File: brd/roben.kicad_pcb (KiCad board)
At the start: 2 copper layers, 47.6 x 90.2 mm, 45 parts, among them J1 POWER IN, J10 1+, J11 1-, J12 2-, J13 2+, J2 +V, J3 GND, J4 +V, J5 GND, J6 A, J7 B, J8 C, J9 D, U1 TPS54232, U2 SN754410N, U3 Ardunano

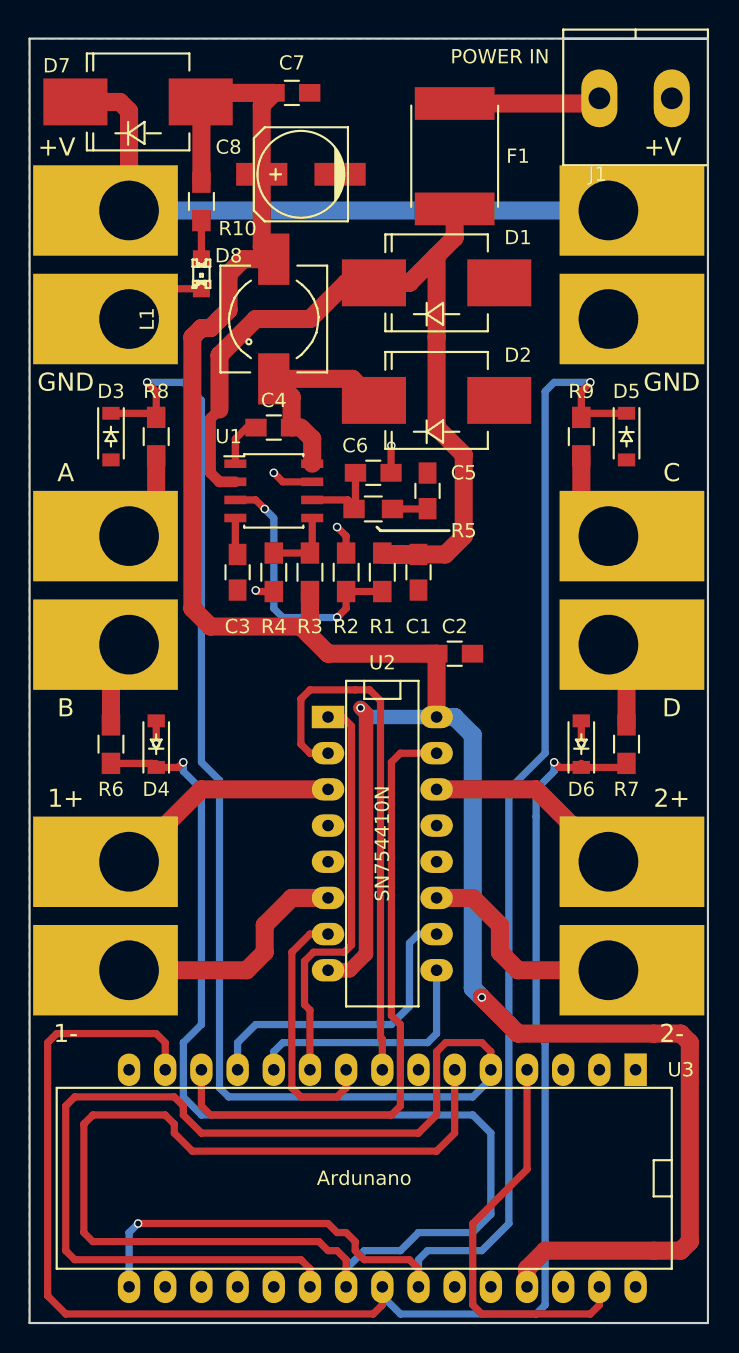
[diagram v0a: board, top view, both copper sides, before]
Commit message: chg: diseñado pcb
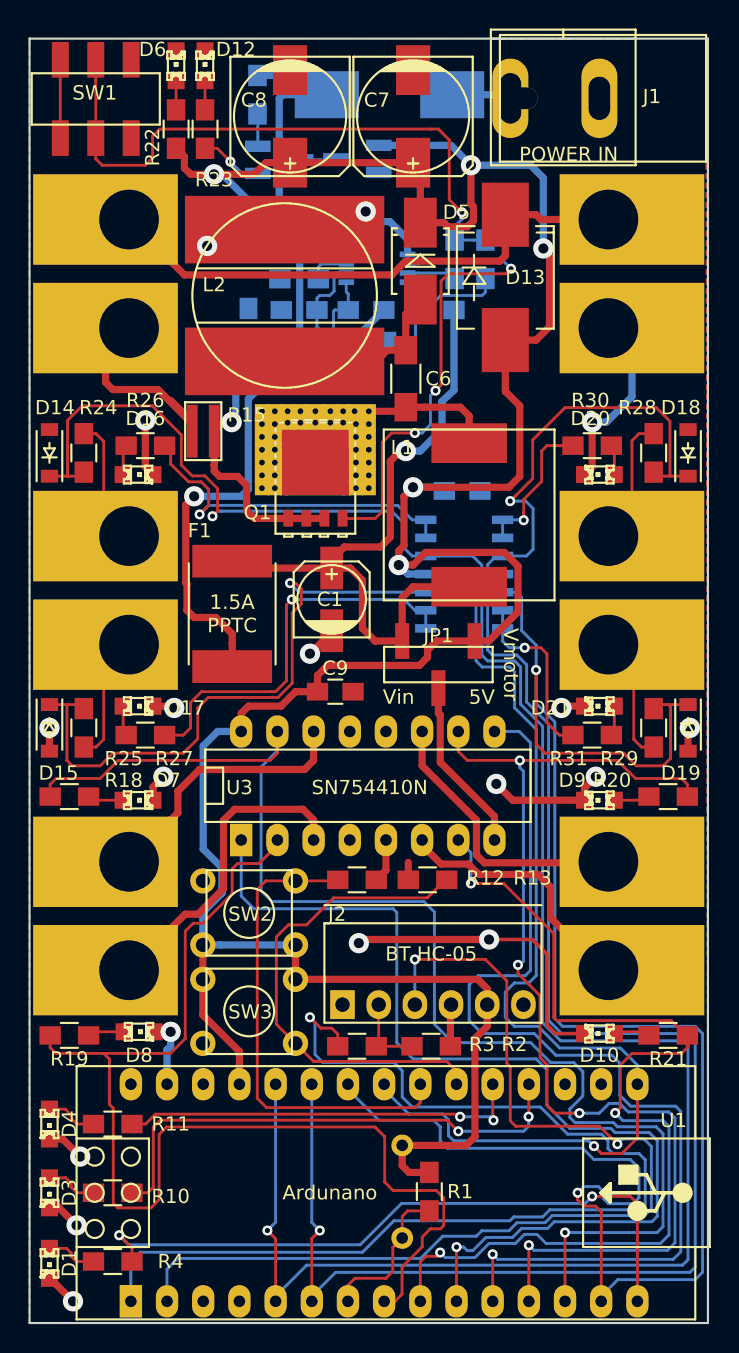
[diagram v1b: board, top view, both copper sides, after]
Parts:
- removed the J7 at (136.5, 93.3)
- removed the J8 at (170.2, 85.7)
- removed the J9 at (170.2, 93.3)
- removed REF**: Symbol_OSHW-Logo_SilkScreen_BIG, Symbols:Symbol_OSHW-Logo_SilkScreen_BIG
- added B: B, Wire_Pads:SolderWirePad_single_2-5mmDrill, F.Cu at (155.6, 81.9)
- added C: C, Wire_Pads:SolderWirePad_single_2-5mmDrill, F.Cu at (153.0, 101.6)
- added C10: 100nF, Capacitors_SMD:C_0805_HandSoldering, B.Cu at (159.9, 82.5)
- added C9: 100nF, Capacitors_SMD:C_0805_HandSoldering, F.Cu at (151.0, 96.6)
- added D: D, Wire_Pads:SolderWirePad_single_2-5mmDrill, F.Cu at (155.6, 111.1)
- added D10: ORANGE, LEDs:LED-0805, F.Cu at (169.5, 120.7)
- added D11: TCMBD914, Housings_SOT-23_SOT-143_TSOT-6:SOT-23_Handsoldering, B.Cu at (152.5, 59.2)
- added D12: ORANGE, LEDs:LED-0805, F.Cu at (141.9, 52.7)
- added D13: B340, Diodes_SMD:Diode-SMC_Handsoldering, F.Cu at (162.9, 67.6)
- added D14: 5V1, Diodes_SMD:SOD-123, F.Cu at (130.9, 79.9)
- added D15: 5V1, Diodes_SMD:SOD-123, F.Cu at (130.9, 99.2)
- added D16: ORANGE, LEDs:LED-0805, F.Cu at (137.2, 81.4)
- added D17: ORANGE, LEDs:LED-0805, F.Cu at (137.2, 97.7)
- added D18: 5V1, Diodes_SMD:SOD-123, F.Cu at (175.8, 79.9)
- added D19: 5V1, Diodes_SMD:SOD-123, F.Cu at (175.8, 99.2)
- added D20: ORANGE, LEDs:LED-0805, F.Cu at (169.5, 81.4)
- added D21: ORANGE, LEDs:LED-0805, F.Cu at (169.5, 97.7)
- added D9: ORANGE, LEDs:LED-0805, F.Cu at (169.5, 104.3)
- added G1: LOGO, asrdi-heatsink:roben, B.Cu at (148.3, 91.7)
- added J2: BT HC-05, asrdi-socket:HC-05, F.Cu at (151.5, 118.6)
- added JP1: VSEL, asrdi-conn:M20-87703xx, F.Cu at (155.7, 93.1)
- added L2: 68uH, asrdi-discrete:coil-13x13H7, F.Cu at (147.4, 68.8)
- added LS1: AT-1224-TWT-5V-2-R, asrdi-buzzer:AT-1224-TWT-5V-2-R, B.Cu at (155.7, 128.5)
- added Q1: BUK7Y98, Power_Packages_SMD:SOT-669_LFPAK_ThermalVias-1, F.Cu at (149.6, 81.7)
- added Q2: BC856, Housings_SOT-23_SOT-143_TSOT-6:SOT-23_Handsoldering, B.Cu at (147.1, 59.3)
- added R11: 220R, Resistors_SMD:R_0805_HandSoldering, F.Cu at (135.4, 127.0)
- added R12: 10k, Resistors_SMD:R_0805_HandSoldering, F.Cu at (152.5, 109.9)
- added R13: 10k, Resistors_SMD:R_0805_HandSoldering, F.Cu at (157.5, 109.9)
- added R14: 100R, Resistors_SMD:R_0805_HandSoldering, B.Cu at (148.5, 74.2)
- added R15: 18m, asrdi-discrete:0612, F.Cu at (141.7, 78.4)
- added R16: 29k4, Resistors_SMD:R_0805_HandSoldering, B.Cu at (148.5, 65.5)
- added R17: 10k, Resistors_SMD:R_0805_HandSoldering, B.Cu at (148.5, 67.7)
- added R18: 220R, Resistors_SMD:R_0805_HandSoldering, F.Cu at (132.3, 104.0)
- added R19: 220R, Resistors_SMD:R_0805_HandSoldering, F.Cu at (132.3, 120.8)
- added R20: 220R, Resistors_SMD:R_0805_HandSoldering, F.Cu at (174.4, 104.0)
- added R21: 220R, Resistors_SMD:R_0805_HandSoldering, F.Cu at (174.4, 120.8)
- added R22: 220R, Resistors_SMD:R_0805_HandSoldering, F.Cu at (139.8, 57.1)
- added R23: 220R, Resistors_SMD:R_0805_HandSoldering, F.Cu at (141.9, 57.1)
- added R24: 220R, Resistors_SMD:R_0805_HandSoldering, F.Cu at (133.3, 79.9)
- added R25: 220R, Resistors_SMD:R_0805_HandSoldering, F.Cu at (133.3, 99.2)
- added R26: 220R, Resistors_SMD:R_0805_HandSoldering, F.Cu at (137.7, 79.4)
- added R27: 220R, Resistors_SMD:R_0805_HandSoldering, F.Cu at (137.7, 99.7)
- added R28: 220R, Resistors_SMD:R_0805_HandSoldering, F.Cu at (173.4, 79.9)
- added R29: 220R, Resistors_SMD:R_0805_HandSoldering, F.Cu at (173.4, 99.2)
- added R30: 220R, Resistors_SMD:R_0805_HandSoldering, F.Cu at (169.0, 79.4)
- added R31: 220R, Resistors_SMD:R_0805_HandSoldering, F.Cu at (169.0, 99.7)
- added SW1: POWER ON, asrdi-switch:JS202011SCQN, F.Cu at (131.7, 57.8)
- added SW2: SW_PUSH, asrdi-switch:FSMxxJxH, F.Cu at (141.7, 109.9)
- added SW3: SW_PUSH, asrdi-switch:FSMxxJxH, F.Cu at (148.2, 121.3)
- added U4: LM2902N, Housings_SOIC:SOIC-14_3.9x8.7mm_Pitch1.27mm, B.Cu at (160.1, 88.4)
- C1: value 4.7uF -> 10uF; footprint Capacitors_SMD:C_0805_HandSoldering -> Capacitors_SMD:c_elec_5x5.3
- C2, D2: moved to B.Cu
- C3: value 8.2nF -> 1.6nF; moved to B.Cu
- C4: value 100nF -> 390nF; moved to B.Cu
- C5: value 390pF -> 2.4nF; moved to B.Cu
- C6: value 7pF -> 4.7uF; footprint Capacitors_SMD:C_0805_HandSoldering -> Capacitors_SMD:C_1206_HandSoldering
- C7: value 22uF -> 470uF; footprint Capacitors_SMD:C_0805_HandSoldering -> Capacitors_SMD:c_elec_8x10
- C8: value 100uF -> 470uF; footprint Capacitors_SMD:c_elec_6.3x5.3 -> Capacitors_SMD:c_elec_8x10
- D1: value B340 -> RED; footprint Diodes_SMD:Diode-SMC_Handsoldering -> LEDs:LED-0805
- D3: value 5V1 -> YELLOW; footprint Diodes_SMD:SOD-123 -> LEDs:LED-0805
- D4: value 5V1 -> GREEN; footprint Diodes_SMD:SOD-123 -> LEDs:LED-0805
- D5: value 5V1 -> SD2114S040S8R0; footprint Diodes_SMD:SOD-123 -> Diodes_SMD:Diode-SMB_Handsoldering
- D6: value 5V1 -> BLUE; footprint Diodes_SMD:SOD-123 -> LEDs:LED-0805
- D7: value B340 -> ORANGE; footprint Diodes_SMD:Diode-SMC_Handsoldering -> LEDs:LED-0805
- D8: value LED -> ORANGE
- F1: value 2A PPTC -> 1.5A PPTC
- J1: footprint asrdi-conn:MKDSN-1985946-02 -> asrdi-conn:combo-barrel5.5x2.1-2p5.08
- L1: value 8.2uH -> 22uH; footprint Choke_SMD:Choke_SMD_Wuerth-WE-PD-Typ-M-Typ-S_Handsoldering -> asrdi-discrete:coil-12x12h10
- R2: value 1M -> 18k
- R4: value 2k -> 220R
- R5: value 63.4k -> 10k; moved to B.Cu
- R6: value 220R -> 20R; moved to B.Cu
- R7: value 220R -> 10k; moved to B.Cu
- R8: value 220R -> 154k; moved to B.Cu
- R9: value 220R -> 1k96; moved to B.Cu
- U1: value TPS54232 -> Ardunano; footprint Housings_SOIC:SOIC-8_3.9x4.9mm_Pitch1.27mm -> asrdi-socket:Ardunano
- U2: value SN754410N -> LM3488; footprint Housings_DIP:DIP-16__300_ELL -> Housings_SSOP:TSSOP-8_3x3mm_Pitch0.65mm; moved to B.Cu
- U3: value Ardunano -> SN754410N; footprint Housings_DIP:DIP-32__600_ELL -> Housings_DIP:DIP-16__300_ELL
- moved D1 74.0 mm to (130.9, 136.8), turned to 90 degrees
- moved R10 69.9 mm to (135.4, 131.8), turned to 0 degrees
- moved D6 55.5 mm to (139.8, 52.7), turned to 270 degrees
- moved D8 53.4 mm to (137.2, 120.5), turned to 180 degrees
- moved D3 53.3 mm to (130.9, 131.8), turned to 90 degrees
- moved U1 50.1 mm to (155.7, 131.8)
- moved R4 49.7 mm to (135.4, 136.7), turned to 180 degrees
- moved D7 49.0 mm to (137.2, 104.3), turned to 180 degrees
- moved R1 43.6 mm to (157.6, 131.7)
- moved U2 40.4 mm to (153.9, 66.9), turned to 0 degrees
- moved R6 38.0 mm to (158.0, 69.8), turned to 180 degrees
- moved F1 35.7 mm to (143.8, 91.2), turned to 90 degrees
- moved R7 35.4 mm to (161.5, 66.3), turned to 90 degrees
- moved R2 33.8 mm to (157.7, 121.5), turned to 0 degrees
- moved R3 33.4 mm to (152.5, 121.5), turned to 180 degrees
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- renumbered J5 to J10, J6 to J11, J10 to J3, J11 to J4, J13 to J5, J12 to J6, J2 to J7, J3 to J8, J4 to J9
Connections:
- C2 pad 1: +5V -> Net-(C2-Pad1)
- C4 pad 2: Net-(C4-Pad2) -> GND
- C6 pad 2: GND -> Net-(C6-Pad2)
- D1 pad 1: Net-(C1-Pad1) -> GND
- D1 pad 2: GND -> Net-(D1-Pad2)
- D2 pad 1: Net-(C4-Pad1) -> Net-(D2-Pad1)
- D2 pad 2: GND -> Net-(D2-Pad2)
- D3 pad 1: Net-(D3-Pad1) -> GND
- D3 pad 2: GND -> Net-(D3-Pad2)
- D4 pad 1: Net-(D4-Pad1) -> GND
- D4 pad 2: GND -> Net-(D4-Pad2)
- D5 pad 1: Net-(D5-Pad1) -> +5V
- D5 pad 2: GND -> Net-(C6-Pad1)
- D6 pad 1: Net-(D6-Pad1) -> GND
- D6 pad 2: GND -> Net-(D6-Pad2)
- D7 pad 1: Net-(D7-Pad1) -> GND
- D7 pad 2: +5V -> Net-(D7-Pad2)
- F1 pad 1: Net-(F1-Pad1) -> Net-(D2-Pad1)
- J1 pad 2: Net-(F1-Pad1) -> Net-(D2-Pad2)
- J11 pad 1: Net-(J6-Pad1) -> Net-(J11-Pad1)
- J3 pad 1: Net-(J10-Pad1) -> Net-(J3-Pad1)
- J4 pad 1: Net-(J11-Pad1) -> Net-(J4-Pad1)
- J5 pad 1: Net-(J13-Pad1) -> Net-(J5-Pad1)
- J6 pad 1: Net-(J12-Pad1) -> Net-(J6-Pad1)
- J7 pad 1: Net-(D7-Pad1) -> Net-(D13-Pad1)
- J9 pad 1: Net-(D7-Pad1) -> Net-(D13-Pad1)
- L1 pad 1: Net-(C4-Pad1) -> Net-(C1-Pad1)
- L1 pad 2: +5V -> Net-(C6-Pad2)
- R1 pad 1: Net-(C1-Pad1) -> +5V
- R1 pad 2: Net-(R1-Pad2) -> Net-(LS1-Pad2)
- R10 pad 1: +5V -> Net-(D3-Pad2)
- R10 pad 2: Net-(D8-Pad2) -> Net-(R10-Pad2)
- R2 pad 1: Net-(R1-Pad2) -> Net-(J2-Pad2)
- R3 pad 1: +5V -> Net-(J2-Pad2)
- R4 pad 1: Net-(R3-Pad2) -> Net-(R4-Pad1)
- R4 pad 2: GND -> Net-(D1-Pad2)
- R5 pad 1: Net-(C6-Pad1) -> Net-(Q2-Pad2)
- R5 pad 2: Net-(C5-Pad1) -> Net-(D2-Pad1)
- R6 pad 1: Net-(J7-Pad1) -> Net-(C1-Pad1)
- R6 pad 2: Net-(D4-Pad1) -> Net-(C2-Pad1)
- R7 pad 1: Net-(J9-Pad1) -> Net-(C2-Pad1)
- R7 pad 2: Net-(D6-Pad1) -> Net-(R7-Pad2)
- R8 pad 1: Net-(J6-Pad1) -> Net-(R8-Pad1)
- R8 pad 2: Net-(D3-Pad1) -> Net-(R7-Pad2)
- R9 pad 1: Net-(J8-Pad1) -> Net-(C3-Pad1)
- R9 pad 2: Net-(D5-Pad1) -> Net-(C4-Pad1)
- U1 pad 1: Net-(C4-Pad2) -> Net-(R3-Pad2)
- U1 pad 2: Net-(C1-Pad1) -> Net-(J2-Pad3)
- U1 pad 3: Net-(R1-Pad2) -> (no net)
- U1 pad 4: Net-(C3-Pad1) -> GND
- U1 pad 5: Net-(R3-Pad2) -> A7
- U1 pad 6: Net-(C6-Pad1) -> A6
- U1 pad 7: GND -> Net-(LS1-Pad2)
- U1 pad 8: Net-(C4-Pad1) -> D5
- U2 pad 1: Net-(U2-Pad1) -> Net-(C5-Pad1)
- U2 pad 2: Net-(U2-Pad2) -> Net-(C3-Pad1)
- U2 pad 3: Net-(J10-Pad1) -> Net-(R16-Pad2)
- U2 pad 6: Net-(J11-Pad1) -> Net-(Q1-Pad4)
- U2 pad 7: Net-(U2-Pad7) -> Net-(R8-Pad1)
- U2 pad 8: +5V -> Net-(C2-Pad1)
- U3 pad 1: Net-(U3-Pad1) -> D7
- U3 pad 10: Net-(U2-Pad1) -> D9
- U3 pad 11: Net-(U2-Pad9) -> Net-(J5-Pad1)
- U3 pad 12: Net-(U2-Pad10) -> GND
- U3 pad 13: Net-(U2-Pad15) -> GND
- U3 pad 14: Net-(D6-Pad1) -> Net-(J3-Pad1)
- U3 pad 15: Net-(U3-Pad15) -> D10
- U3 pad 16: Net-(D5-Pad1) -> +5V
- U3 pad 2: Net-(U3-Pad2) -> D5
- U3 pad 3: Net-(U3-Pad3) -> Net-(J4-Pad1)
- U3 pad 5: Net-(D3-Pad1) -> GND
- U3 pad 6: Net-(D4-Pad1) -> Net-(J6-Pad1)
- U3 pad 7: Net-(U3-Pad7) -> D6
- U3 pad 8: Net-(U2-Pad2) -> VCOM
- U3 pad 9: Net-(U2-Pad7) -> D8
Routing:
- net A7: track 0.00 -> 152.1 mm, vias 0 -> 2
- net Net-(D3-Pad1): track 147.0 -> 0.00 mm, vias 1 -> 0
- net A6: track 0.00 -> 136.4 mm, vias 0 -> 2
- net Net-(D4-Pad1): track 133.1 -> 0.00 mm, vias 1 -> 0
- net A5: track 0.00 -> 129.6 mm, vias 0 -> 2
- net A4: track 0.00 -> 118.7 mm, vias 0 -> 2
- net Net-(D6-Pad1): track 111.5 -> 0.00 mm, vias 1 -> 0
- net Net-(D5-Pad1): track 105.6 -> 0.00 mm, vias 2 -> 0
- net D10: track 0.00 -> 93.1 mm, vias 0 -> 1
- net D5: track 0.00 -> 82.1 mm
- net D9: track 0.00 -> 78.6 mm, vias 0 -> 4
- net Net-(J2-Pad3): track 0.00 -> 73.9 mm, vias 0 -> 2
- net Net-(R3-Pad2): track 5.07 -> 77.8 mm, vias 0 -> 1
- net D8: track 0.00 -> 72.3 mm, vias 0 -> 1
- net D7: track 0.00 -> 71.4 mm, vias 0 -> 1
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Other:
- net class Default: clearance 0.2 -> 0.2032; trace_width 0.25 -> 0.2032; via_dia 0.6 -> 0.7112; via_drill 0.4 -> 0.3556
- net class Power added: clearance 0.2032, trace_width 0.508, via_dia 1.4224, via_drill 0.7112
- rule trace_clearance: 0.2 -> 0.2032
- board text added: "+"
- board text added: "-"
- board text added: "1.5A PPTC"
- board text added: "5V"
- board text added: "OFF"
- board text added: "ON"
- board text added: "Released under GNU/GPL 3 License https://www.gnu.org/licenses/gpl.html Copyright (C) 2015-2016 kwendenarmo https://github.com/akornsys-rdi/robgednaut"
- board text added: "Roben Zond"
- board text added: "Vin 3-32V"
- board text added: "Vmotor"
- board text added: "v2.0.0"
- board text removed: "+V"
- board text removed: "1+"
- board text removed: "1-"
- board text removed: "2+"
- board text removed: "2-"
- board text removed: "A"
- board text removed: "B"
- board text removed: "C"
- board text removed: "D"
- board text removed: "GND"
- board text removed: "Released under GNU/GPL 3 License https://www.gnu.org/licenses/gpl.html Copyright (C) 2015 kwendenarmo https://github.com/akornsys-rdi/robgednaut"
- board text removed: "Roben"
- board text removed: "v1.0.0"
